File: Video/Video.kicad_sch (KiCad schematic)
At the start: 1 part

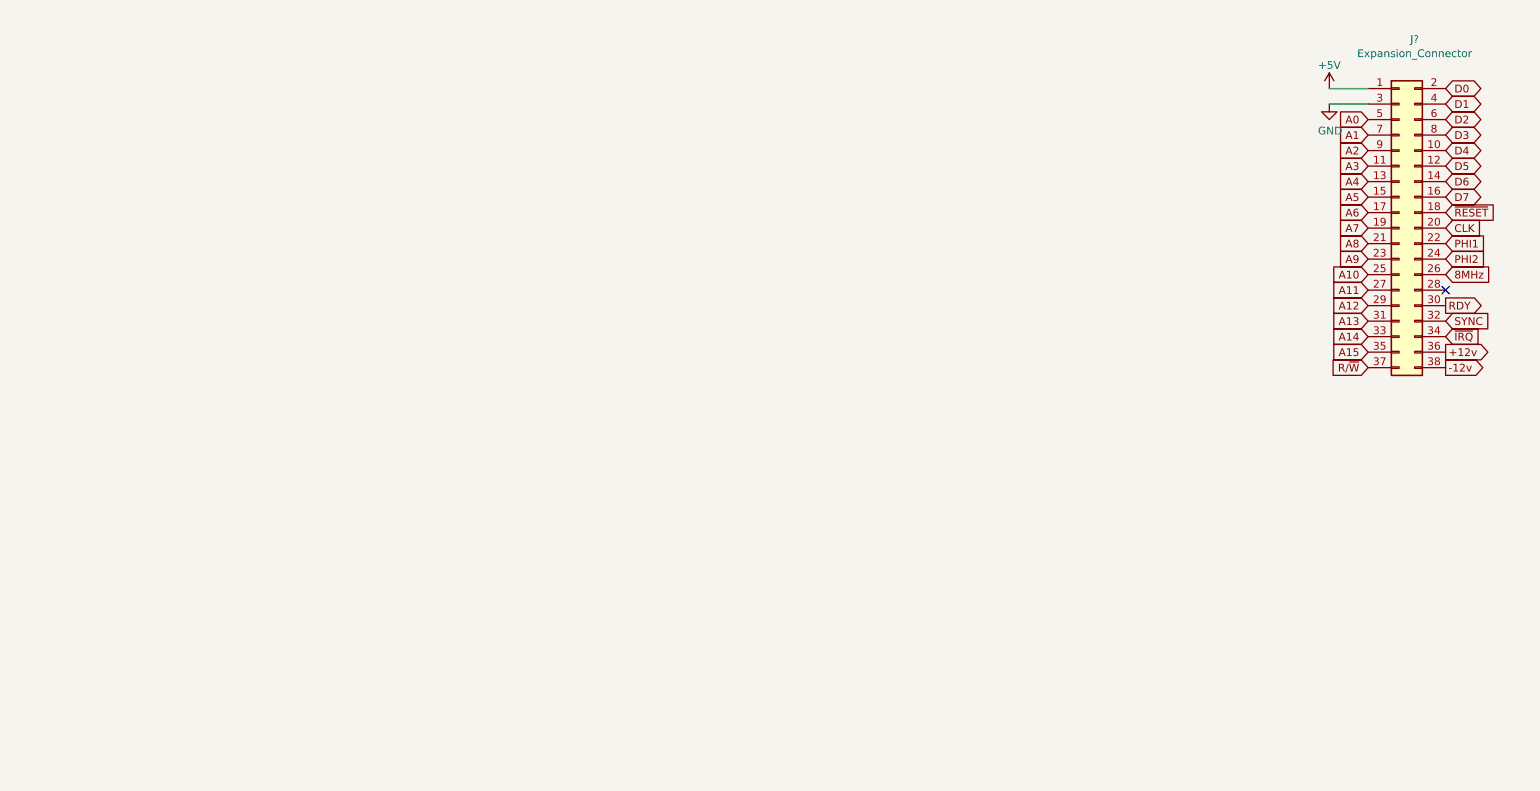
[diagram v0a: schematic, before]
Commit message: Video card added...
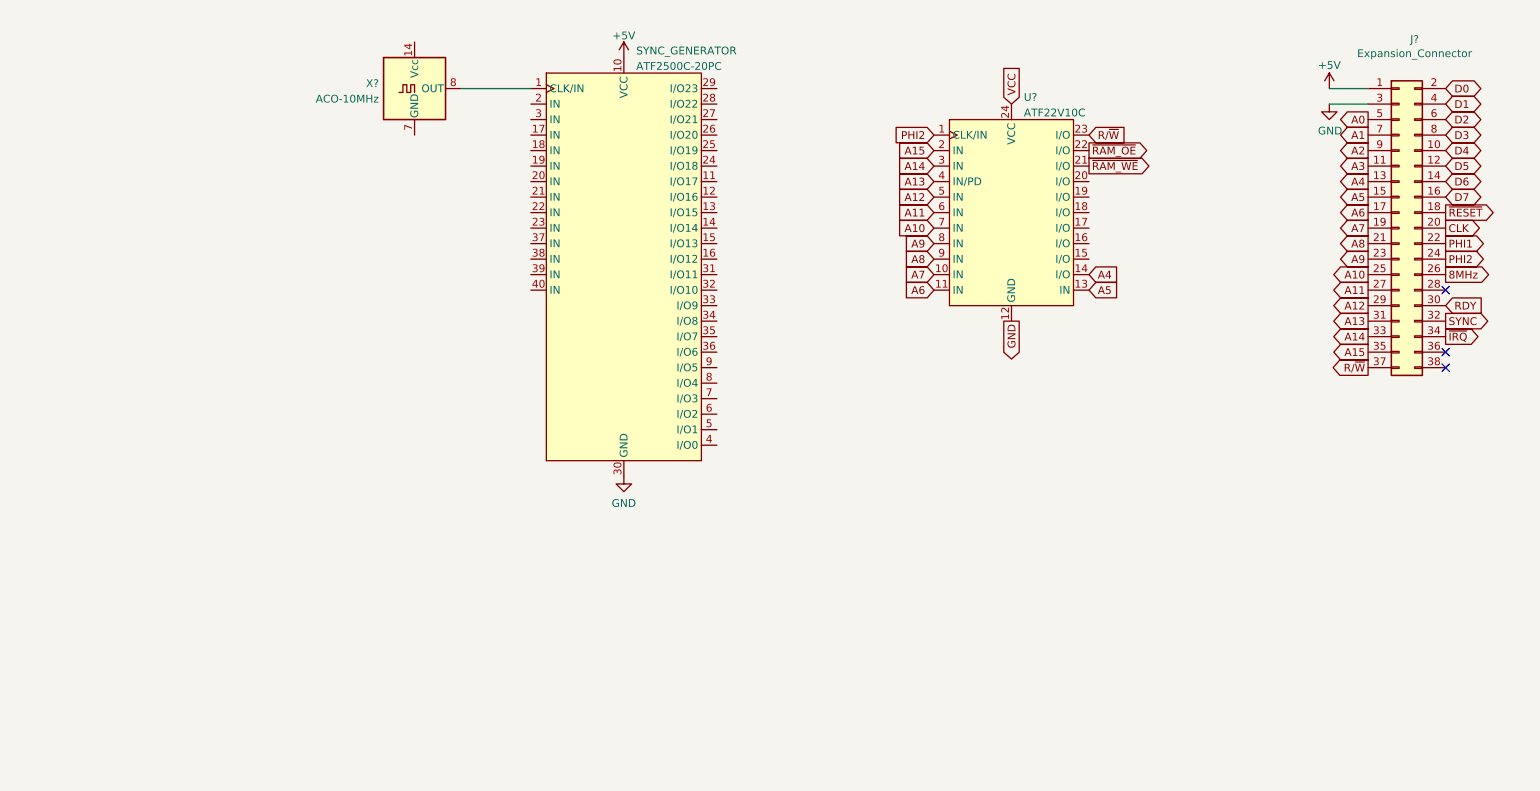
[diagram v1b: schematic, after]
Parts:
- added SYNC_GENERATOR: ATF2500C-20PC, symbol PC:ATF2500C-40P6
- added U?: ATF22V10C, Package_DIP:DIP-24_W7.62mm_Socket_LongPads, symbol PC:ATF22V10C
- added X?: ACO-10MHz, Oscillator:Oscillator_DIP-14, symbol Oscillator:ACO-xxxMHz
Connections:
- net +5V: now also SYNC_GENERATOR.10 (VCC)
- net A10: now also U?.7 (IN)
- net A11: now also U?.6 (IN)
- net A12: now also U?.5 (IN)
- net A13: now also U?.4 (IN/PD)
- net A14: now also U?.3 (IN)
- net A15: now also U?.2 (IN)
- net A4: now also U?.14 (I/O)
- net A5: now also U?.13 (IN)
- net A6: now also U?.11 (IN)
- net A7: now also U?.10 (IN)
- net A8: now also U?.9 (IN)
- net A9: now also U?.8 (IN)
- net GND: now also SYNC_GENERATOR.30 (GND), U?.12 (GND)
- net PHI2: now also U?.1 (CLK/IN)
- net R/~{W}: now also U?.23 (I/O)
- net +12v: no longer names the net of J?.36 (Pin_36)
- net -12v: no longer names the net of J?.38 (Pin_38)
- new net: SYNC_GENERATOR.1 (CLK/IN), X?.8 (OUT)
- new net VCC: U?.24 (VCC)
- new net ~{RAM_OE}: U?.22 (I/O)
- new net ~{RAM_WE}: U?.21 (I/O)
- no-connect marks 1 -> 3

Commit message: Added components...
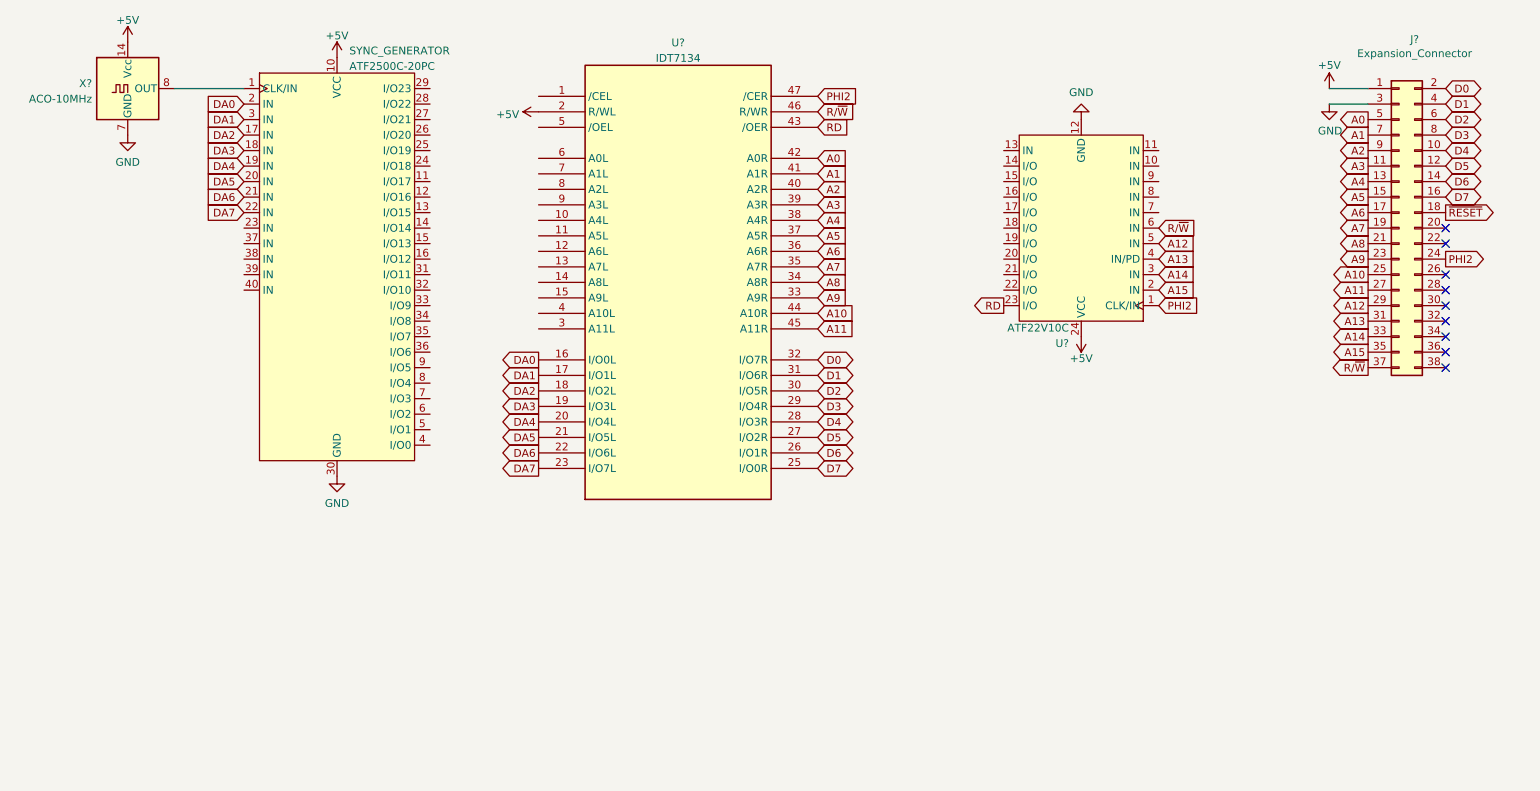
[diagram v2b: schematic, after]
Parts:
- added U?: IDT7134, symbol PC:IDT7134
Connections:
- net +5V: now also U?.24 (VCC), X?.14 (Vcc), U?.2 (R/WL)
- net A0: now also U?.42 (A0R)
- net A1: now also U?.41 (A1R)
- net A10: now also U?.44 (A10R); no longer U?.7 (IN)
- net A11: now also U?.45 (A11R); no longer U?.6 (IN)
- net A2: now also U?.40 (A2R)
- net A3: now also U?.39 (A3R)
- net A4: now also U?.38 (A4R); no longer U?.14 (I/O)
- net A5: now also U?.37 (A5R); no longer U?.13 (IN)
- net A6: now also U?.36 (A6R); no longer U?.11 (IN)
- net A7: now also U?.35 (A7R); no longer U?.10 (IN)
- net A8: now also U?.34 (A8R); no longer U?.9 (IN)
- net A9: now also U?.33 (A9R); no longer U?.8 (IN)
- net D0: now also U?.32 (I/O7R)
- net D1: now also U?.31 (I/O6R)
- net D2: now also U?.30 (I/O5R)
- net D3: now also U?.29 (I/O4R)
- net D4: now also U?.28 (I/O3R)
- net D5: now also U?.27 (I/O2R)
- net D6: now also U?.26 (I/O1R)
- net D7: now also U?.25 (I/O0R)
- net GND: now also X?.7 (GND), U?.24 (GND)
- net PHI2: now also U?.47 (/CER)
- net R/~{W}: now also U?.6 (IN), U?.46 (R/WR); no longer U?.23 (I/O)
- net VCC: now also U?.48 (VCC); no longer U?.24 (VCC)
- net DA2: now reaches SYNC_GENERATOR.17 (IN)
- net DA2: now also U?.18 (I/O2L)
- net DA3: now reaches SYNC_GENERATOR.18 (IN)
- net DA3: now also U?.19 (I/O3L)
- net DA4: now reaches SYNC_GENERATOR.19 (IN)
- net DA4: now also U?.20 (I/O4L)
- net DA0: now reaches SYNC_GENERATOR.2 (IN)
- net DA0: now also U?.16 (I/O0L)
- net DA5: now reaches SYNC_GENERATOR.20 (IN)
- net DA5: now also U?.21 (I/O5L)
- net DA6: now reaches SYNC_GENERATOR.21 (IN)
- net DA6: now also U?.22 (I/O6L)
- net DA7: now reaches SYNC_GENERATOR.22 (IN)
- net DA7: now also U?.23 (I/O7L)
- net DA1: now reaches SYNC_GENERATOR.3 (IN)
- net DA1: now also U?.17 (I/O1L)
- net 8MHz: no longer names the net of J?.26 (Pin_26)
- net CLK: no longer names the net of J?.20 (Pin_20)
- net PHI1: no longer names the net of J?.22 (Pin_22)
- net RDY: no longer names the net of J?.30 (Pin_30)
- net SYNC: no longer names the net of J?.32 (Pin_32)
- net ~{IRQ}: no longer names the net of J?.34 (Pin_34)
- net ~{RAM_OE}: no longer names the net of U?.22 (I/O)
- net ~{RAM_WE}: no longer names the net of U?.21 (I/O)
- new net RD: U?.23 (I/O), U?.43 (/OER)
- no-connect marks 3 -> 9
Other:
- moved on the sheet: SYNC_GENERATOR, U?, X?

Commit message: Added reference files...
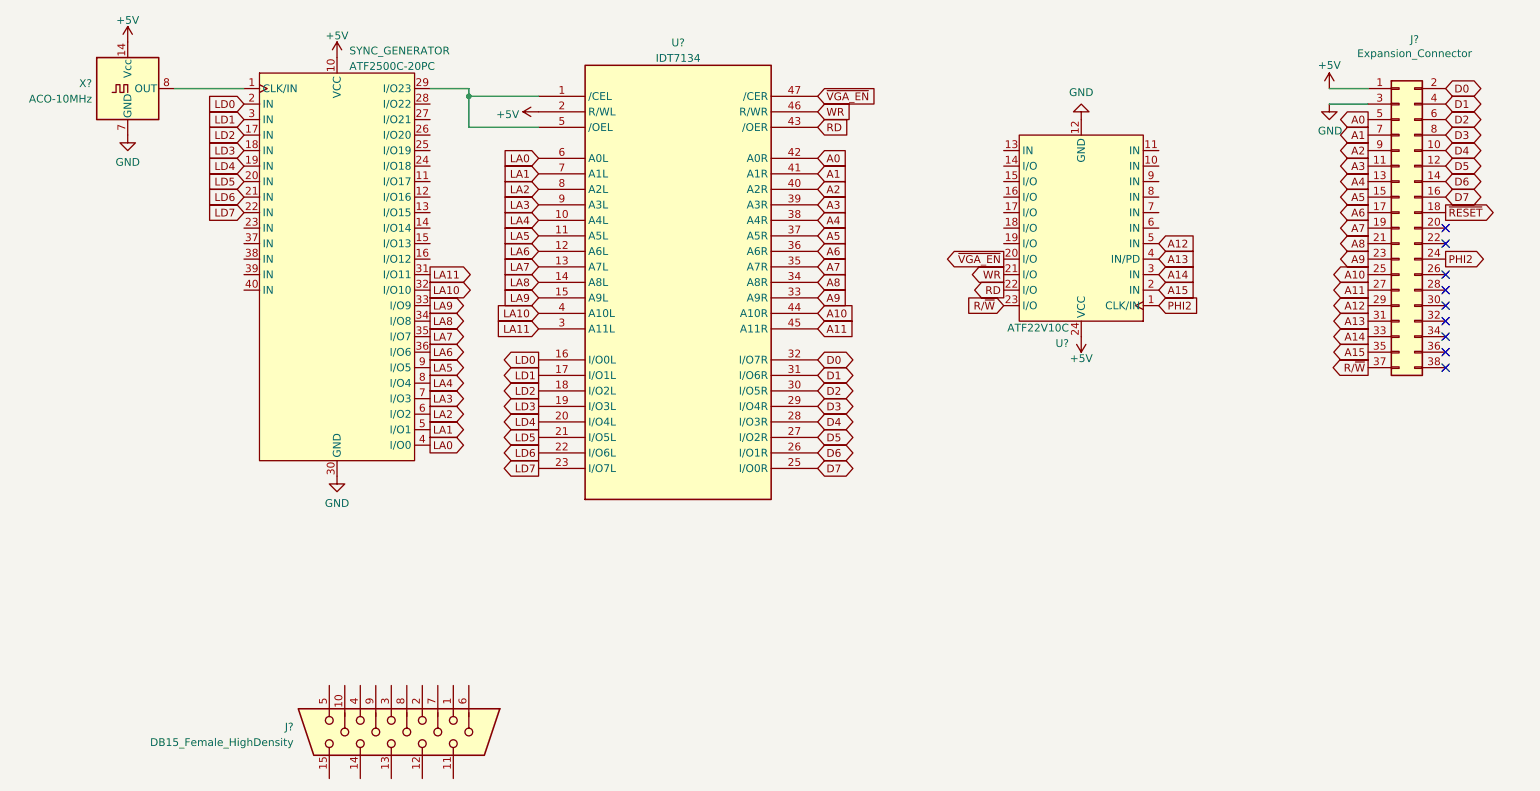
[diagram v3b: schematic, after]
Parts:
- added J?: DB15_Female_HighDensity, symbol Connector:DB15_Female_HighDensity
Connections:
- net PHI2: no longer U?.47 (/CER)
- net RD: now also U?.22 (I/O); no longer U?.23 (I/O)
- net R/~{W}: now also U?.23 (I/O); no longer U?.46 (R/WR), U?.6 (IN)
- net at SYNC_GENERATOR.29 (I/O23): now also U?.1 (/CEL), U?.5 (/OEL)
- net LA11: now reaches SYNC_GENERATOR.31 (I/O11)
- net LA11: now also U?.3 (A11L)
- net LA10: now reaches SYNC_GENERATOR.32 (I/O10)
- net LA10: now also U?.4 (A10L)
- net LA9: now reaches SYNC_GENERATOR.33 (I/O9)
- net LA9: now also U?.15 (A9L)
- net LA8: now reaches SYNC_GENERATOR.34 (I/O8)
- net LA8: now also U?.14 (A8L)
- net LA7: now reaches SYNC_GENERATOR.35 (I/O7)
- net LA7: now also U?.13 (A7L)
- net LA6: now reaches SYNC_GENERATOR.36 (I/O6)
- net LA6: now also U?.12 (A6L)
- net LA0: now reaches SYNC_GENERATOR.4 (I/O0)
- net LA0: now also U?.6 (A0L)
- net LA1: now reaches SYNC_GENERATOR.5 (I/O1)
- net LA1: now also U?.7 (A1L)
- net LA2: now reaches SYNC_GENERATOR.6 (I/O2)
- net LA2: now also U?.8 (A2L)
- net LA3: now reaches SYNC_GENERATOR.7 (I/O3)
- net LA3: now also U?.9 (A3L)
- net LA4: now reaches SYNC_GENERATOR.8 (I/O4)
- net LA4: now also U?.10 (A4L)
- net LA5: now reaches SYNC_GENERATOR.9 (I/O5)
- net LA5: now also U?.11 (A5L)
- net ~{VGA_EN}: now reaches U?.20 (I/O)
- net ~{VGA_EN}: now also U?.47 (/CER)
- net WR: now reaches U?.21 (I/O)
- net WR: now also U?.46 (R/WR)
- net DA0 renamed LD0
- net DA1 renamed LD1
- net DA2 renamed LD2
- net DA3 renamed LD3
- net DA4 renamed LD4
- net DA5 renamed LD5
- net DA6 renamed LD6
- net DA7 renamed LD7
